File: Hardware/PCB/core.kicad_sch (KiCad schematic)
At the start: 26 parts, among them IC3 ATxmega32A4U-A, IC4 741G126DBVAHC, J2 OUT0, Q1 BC817-40W, Q2 NTF2955T1G, U1 ID-12/20SMD

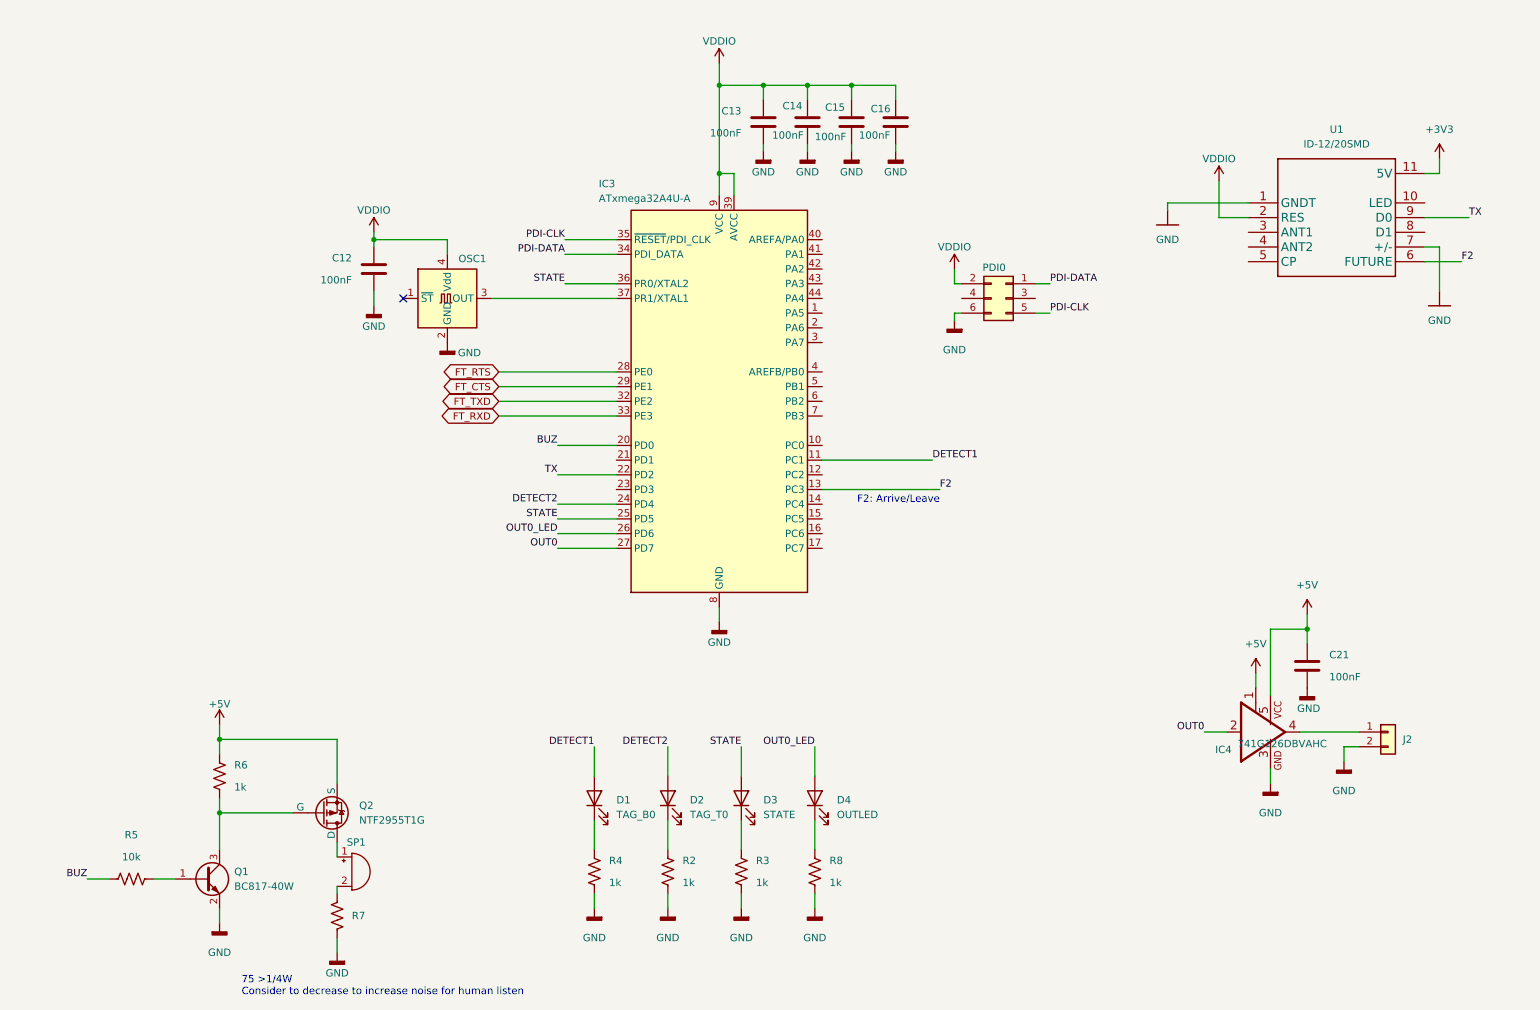
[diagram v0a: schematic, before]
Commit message: versão 1.3 final & ficheiros de manufacturing
- ainda sem revisão do Filipe
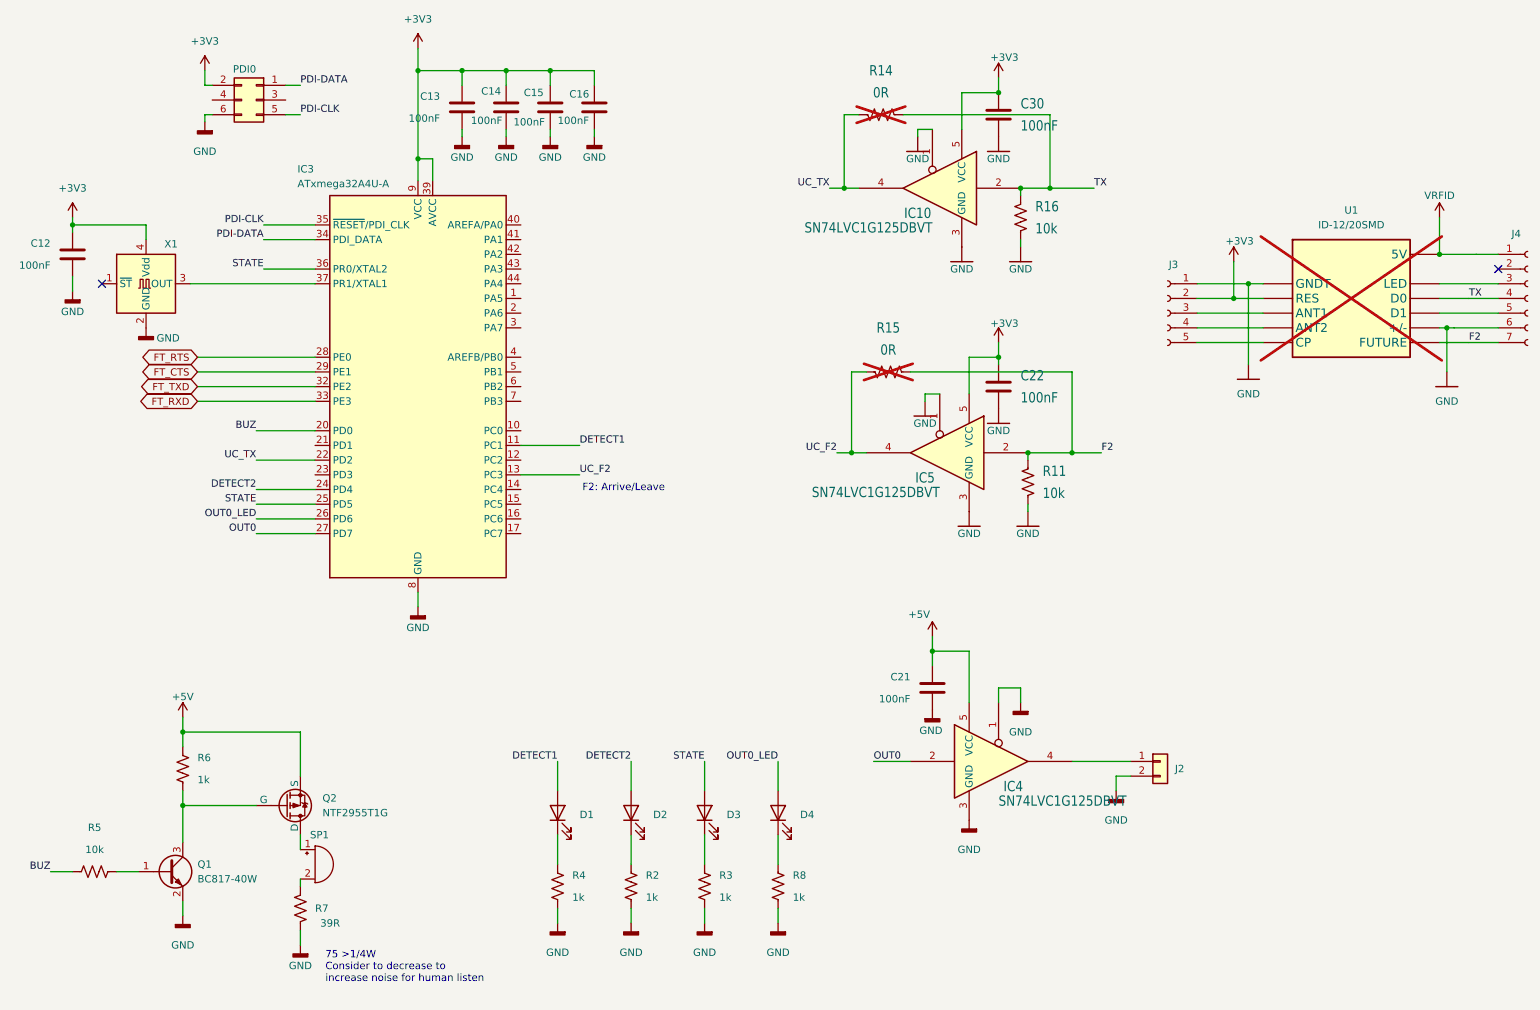
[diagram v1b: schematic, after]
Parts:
- removed IC4: 741G126DBVAHC, Package_TO_SOT_SMD:SOT-23-5, symbol harp rfid reader:741G126DBV
- added C22, C30: 100nF, Capacitor_SMD:C_0402_1005Metric, symbol Device:C
- added IC10, IC4, IC5: SN74LVC1G125DBVT, Package_TO_SOT_SMD:SOT-23-5, symbol 74xGxx:SN74LVC1G125DBV
- added J3: NPPN051BFLD-RC, Connector_PinSocket_2.00mm:PinSocket_1x05_P2.00mm_Vertical_SMD_Pin1Right, symbol Connector:Conn_01x05_Socket
- added J4: NPPN071BFLC-RC, Connector_PinSocket_2.00mm:PinSocket_1x07_P2.00mm_Vertical_SMD_Pin1Right, symbol Connector:Conn_01x07_Socket
- added R11, R16: 10k, Resistor_SMD:R_0402_1005Metric, symbol Device:R_US
- added R14, R15: 0R, Resistor_SMD:R_0402_1005Metric, symbol Device:R_US
- C12, C13, C14, C15, C16, C21: OEPSPN (none) -> OEPS010016; TempCo (none) -> X7R; Tolerance (none) -> ±10%; Voltage (none) -> 50V
- D1: value TAG_B0 -> 5975004407F; OEPSPN (none) -> OEPS030006
- D2: value TAG_T0 -> 5975004407F; OEPSPN (none) -> OEPS030006
- D3: value STATE -> 5975004407F; OEPSPN (none) -> OEPS030006
- D4: value OUTLED -> 5975004407F; OEPSPN (none) -> OEPS030006
- IC3: MPN DNI ????? -> ATXMEGA32A4U-A; OEPSPN (none) -> OEPS080012
- J2: value OUT0 -> 282834-2
- PDI0: value MA03-2 -> 67996-206HLF; MPN (none) -> 67996-206HLF; OEPSPN (none) -> OEPS070015
- Q1: MPN BC817-40W-7 -> BC817-40W-7; OEPSPN (none) -> OEPS060005; Voltage (none) -> 45V
- Q2: Voltage (none) -> 60V
- R2, R3, R4, R6, R8: OEPSPN (none) -> OEPS020027; Tolerance (none) -> ±1%
- R5: OEPSPN (none) -> OEPS020030; Tolerance (none) -> ±1%
- R7: value 75 >1/4W -> 39R; OEPSPN (none) -> OEPS020034; Tolerance (none) -> ±1%
- SP1: value BUZZER-COIL_SMT-0540-S-R -> SMT-0540-S-R; OEPSPN (none) -> OEPS100012
- U1: footprint harp rfid reader:ID-12_SMD -> harp rfid reader:ID-12_SMD body; MPN (none) -> ID-12LA; OEPSPN (none) -> OEPS100013; now not fitted; now left out of the parts list
- X1: renamed from OSC1; value CNP-MISCELLANEOUS_OSCILLATOR -> O 32,0-JT32C-A-K-3,3-LF; MPN O 32,0-JT32C-A-K-3,3-LF -> O 32,0-JT32C-A-K-3,3-LF; OEPSPN (none) -> OEPS080014
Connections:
- net VDDIO is gone; now on net +3V3: C12.1, C13.1, C14.1, C15.1, C16.1, IC3.19 (VCC), IC3.31 (VCC), IC3.39 (AVCC), IC3.9 (VCC), PDI0.2 (Pin_2), U1.2 (RES), X1.4 (Vdd)
- net +3V3: now also C22.1, C30.1, IC10.5 (VCC), IC5.5 (VCC), J3.2 (Pin_2); no longer U1.11 (5V)
- net +5V: now also IC4.5 (VCC)
- net F2: now also IC5.2, J4.7 (Pin_7), R11.1, R15.2; no longer IC3.13 (PC3)
- net GND: now also C22.2, C30.2, IC10.1, IC10.3 (GND), IC4.1, IC4.3 (GND), IC5.1, IC5.3 (GND), J3.1 (Pin_1), J4.6 (Pin_6), R11.2, R16.2
- net OUT0: now also IC4.2
- net TX: now also IC10.2, J4.4 (Pin_4), R14.2, R16.1; no longer IC3.22 (PD2)
- net at J2.1 (Pin_1): now also IC4.4
- net at U1.10 (LED): now also J4.3 (Pin_3)
- net at U1.3 (ANT1): now also J3.3 (Pin_3)
- net at U1.4 (ANT2): now also J3.4 (Pin_4)
- net at U1.5 (CP): now also J3.5 (Pin_5)
- net at U1.8 (D1): now also J4.5 (Pin_5)
- new net UC_F2: IC3.13 (PC3), IC5.4, R15.1
- new net UC_TX: IC10.4, IC3.22 (PD2), R14.1
- new net VRFID: J4.1 (Pin_1), U1.11 (5V)
- no-connect marks 1 -> 2
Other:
- moved on the sheet: C12, C13, C14, C15, C16, C21, D1, D2, D3, D4, IC3, J2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
